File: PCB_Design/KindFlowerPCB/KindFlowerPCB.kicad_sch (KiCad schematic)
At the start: 13 parts, among them J1 LiPo_Connector, J2 FSR_1, J3 Wireless_Charger, J4 FSR_2, J5 FSR_3, J6 FSR_0, J7 NeopixelStrip1, J8 NeopixelStrip2

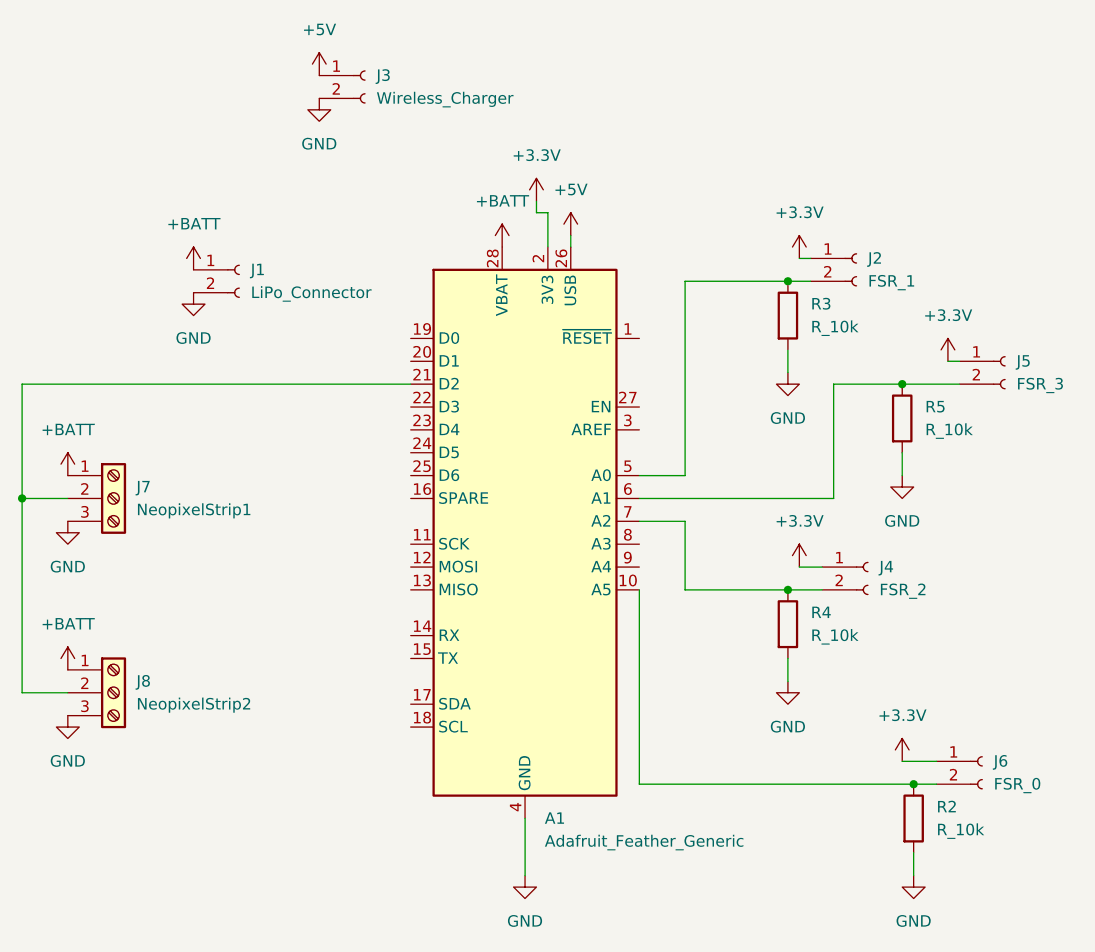
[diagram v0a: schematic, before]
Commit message: Updated PCB files
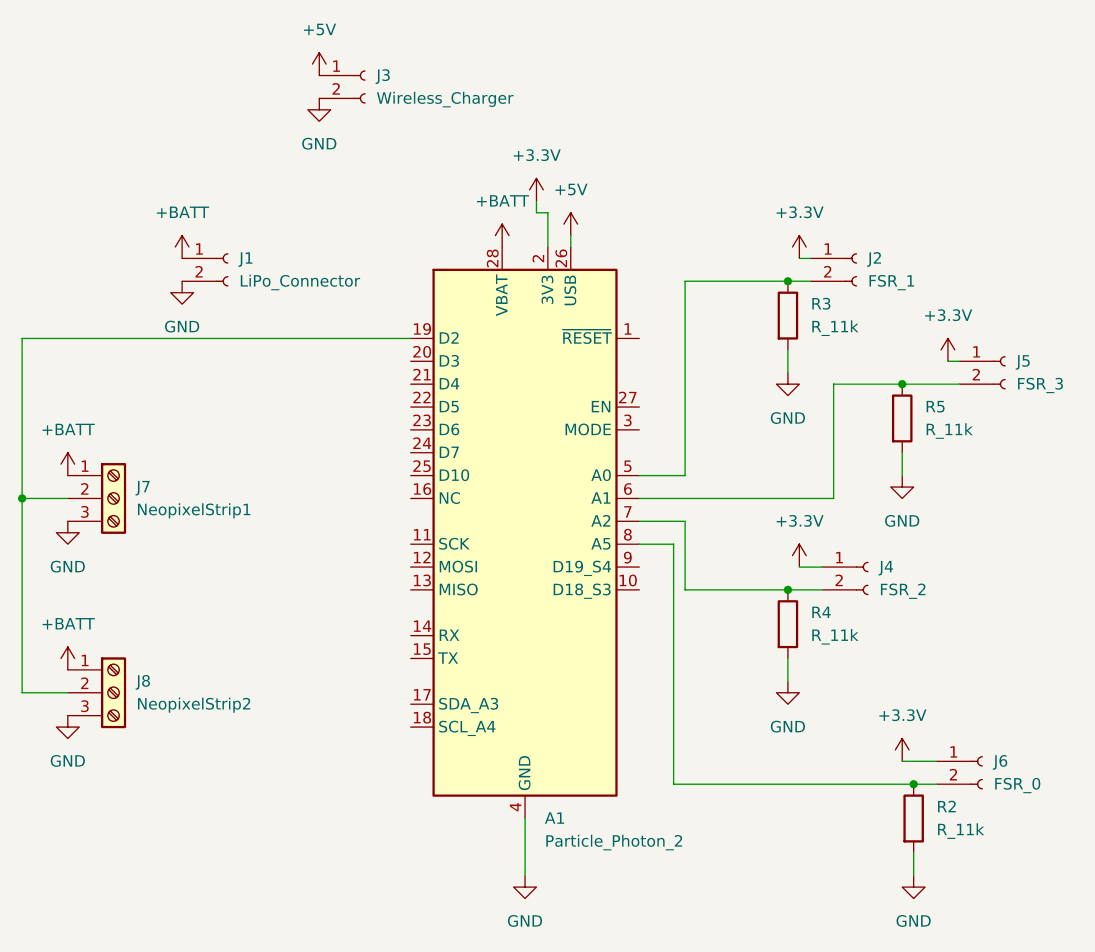
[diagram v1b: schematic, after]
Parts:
- A1: value Adafruit_Feather_Generic -> Particle_Photon_2; footprint Module:Adafruit_Feather -> ParticleBoards:Photon_2; symbol MCU_Module:Adafruit_Feather_Generic -> ParticlePhoton2:Photon_2
- R2, R3, R4, R5: value R_10k -> R_11k
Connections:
- net at J6.2 (Pin_2), R2.1: now also A1.8 (A5); no longer A1.10 (A5)
- net at J7.2 (Pin_2), J8.2 (Pin_2): now also A1.19 (D2); no longer A1.21 (D2)
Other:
- moved on the sheet: J1
